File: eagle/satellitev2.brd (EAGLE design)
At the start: 85.1 x 49.5 mm, 12 parts, among them J1 RJ11-6PTH

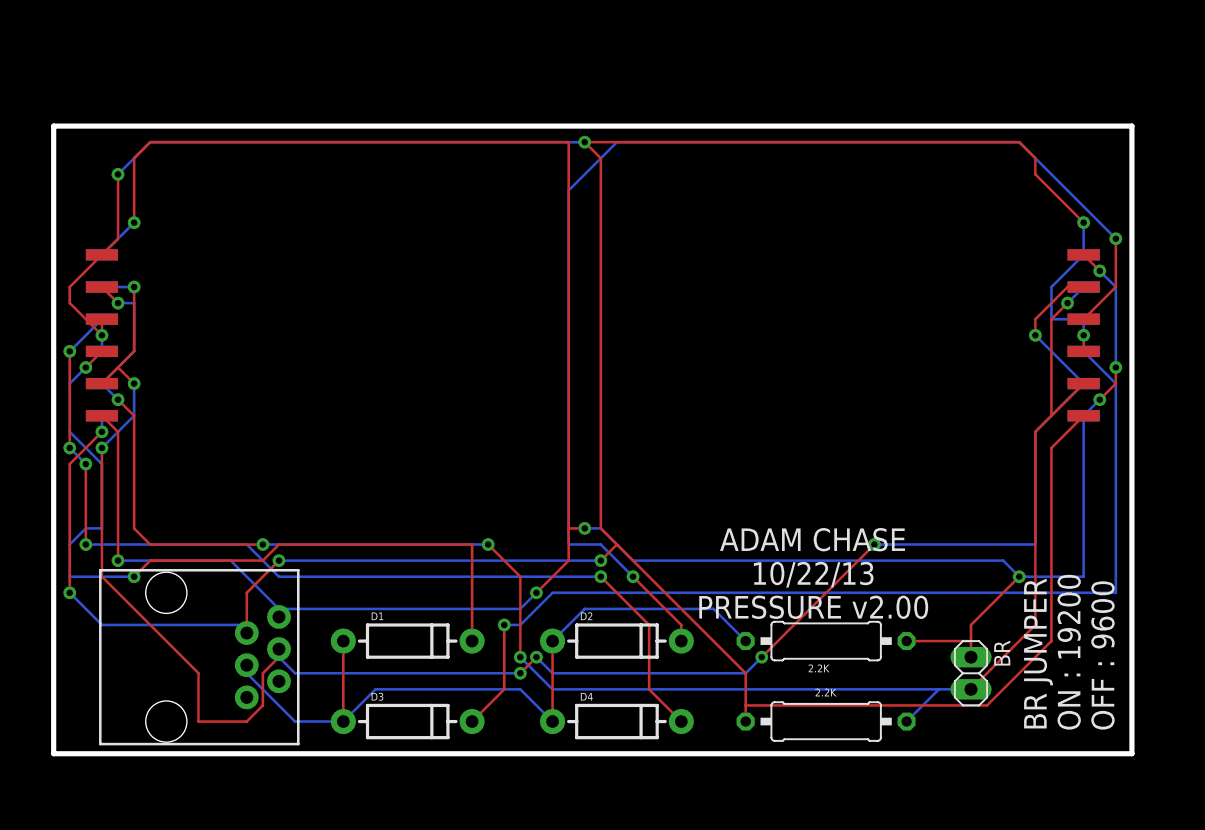
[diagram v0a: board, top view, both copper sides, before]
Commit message: in middle of writing for AIAA paper
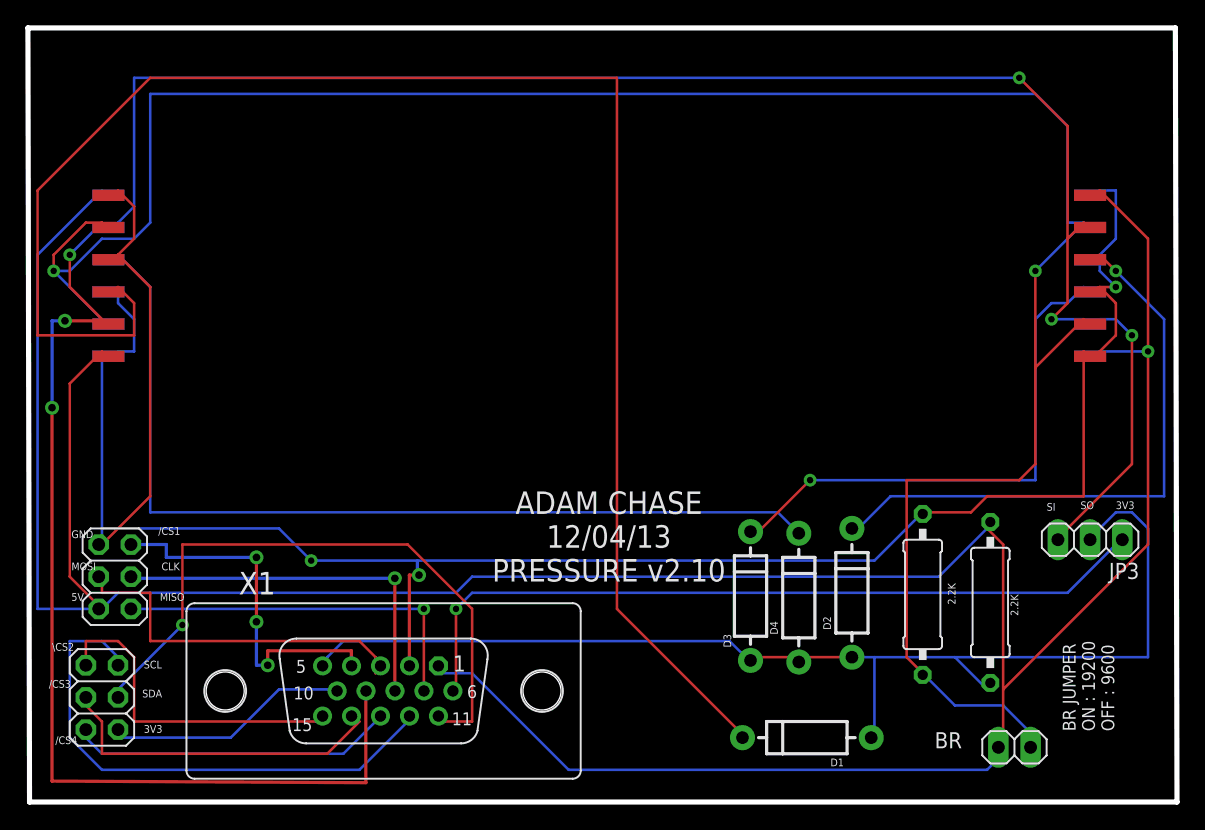
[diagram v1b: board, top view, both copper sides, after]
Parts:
- removed J1: RJ11-6PTH, SparkFun-Connectors:RJ11-6
- added JP1, JP2: (no value), pinhead:2X03
- added JP3: (no value), pinhead:1X03
- added X1: (no value), con-subd:HDF15V
- moved D1 32.4 mm to (59.4, 1.27), turned to 180 degrees
- moved D3 28.8 mm to (55.0, 12.4), turned to 90 degrees
- moved D2 18.9 mm to (63.0, 12.7), turned to 90 degrees
- moved D4 17.4 mm to (58.8, 12.3), turned to 90 degrees
- moved R1 13.3 mm to (73.9, 11.9), turned to 270 degrees
- moved R2 12.6 mm to (68.6, 12.6), turned to 270 degrees
- moved BR 6.77 mm to (75.8, 0.51), turned to 0 degrees
- moved U$1 4.73 mm to (4.32, 44.1)
- moved U$2 4.73 mm to (81.8, 44.1)
- moved U$3 4.73 mm to (80.5, 44.1)
- moved U$4 4.73 mm to (3.05, 44.1)
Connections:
- new net 3V3: JP3.1, X1.6
- new net ACCEL2CS: JP1.5, X1.4
- new net D46: JP2.2, X1.13
- new net D47: JP2.4, X1.14
- new net D48: JP2.6, X1.15
- new net MISO: JP1.1, X1.7
- new net MOSI: JP1.4, X1.3
- new net SCL: JP2.5, X1.12
- new net SCLK: JP1.3, X1.8
- new net SDA: JP2.3, X1.11
- new net TEMPBUS: JP2.1, X1.10
- net 5V: now also JP1.2, X1.1; no longer J1.1
- net GND: now also JP1.6, X1.2; no longer J1.2
- net RX: now also JP3.3, X1.9; no longer J1.3
- net TX: now also JP3.2, X1.5; no longer J1.4
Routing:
- net GND: track 272.9 -> 181.2 mm, vias 9 -> 3
- net RX: track 146.4 -> 215.9 mm, vias 8 -> 6
- net N$2: track 62.1 -> 130.2 mm, vias 2 -> 0
- net 3V3: track 0.00 -> 61.4 mm, vias 0 -> 1
- net SDA: track 0.00 -> 51.0 mm, vias 0 -> 1
- net N$1: track 96.0 -> 47.7 mm, vias 2 -> 1
- net 5V: track 210.5 -> 256.2 mm, vias 8 -> 1
- net SCL: track 0.00 -> 42.3 mm
- net BR: track 140.6 -> 180.3 mm, vias 6 -> 2
- net N$4: track 78.1 -> 42.3 mm
- net TX: track 58.5 -> 93.9 mm
- net SCLK: track 0.00 -> 29.9 mm, vias 0 -> 1
- net MISO: track 0.00 -> 29.6 mm, vias 0 -> 1
- net MOSI: track 0.00 -> 29.4 mm
- net ACCEL2CS: track 0.00 -> 29.3 mm, vias 0 -> 3
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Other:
- board size 85.1 x 49.5 mm -> 90.7 x 61.1 mm
- board text added: "/CS1"
- board text added: "/CS3"
- board text added: "/CS4"
- board text added: "3V3"
- board text added: "ADAM CHASE 12/04/13 PRESSURE v2.10"
- board text added: "CLK"
- board text added: "MISO"
- board text added: "MOSI"
- board text added: "SCL"
- board text added: "SDA"
- board text added: "\CS2"
- board text removed: "ADAM CHASE 10/22/13 PRESSURE v2.00"

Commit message: modified eagle boards and ordered.
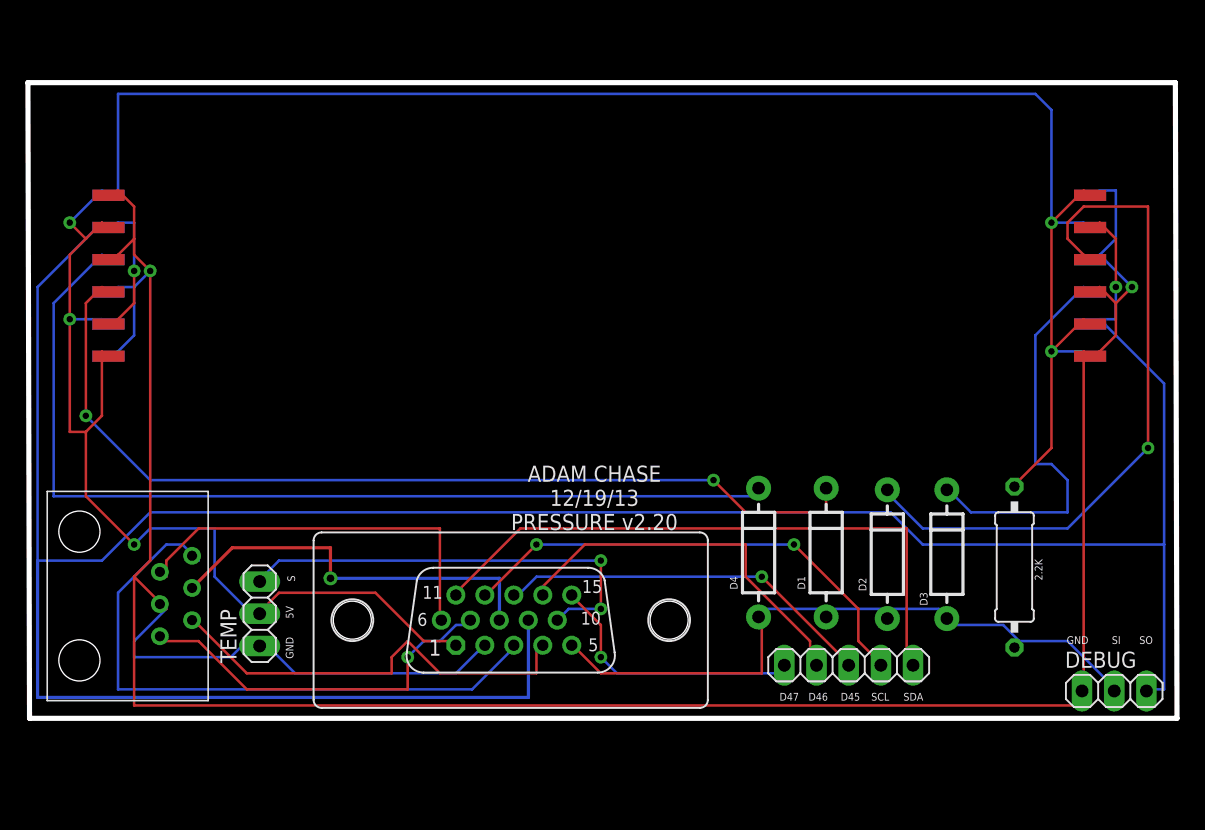
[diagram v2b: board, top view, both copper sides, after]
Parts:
- removed BR: (no value), pinhead:1X02
- removed JP2: (no value), pinhead:2X03
- removed JP3: (no value), pinhead:1X03
- removed R2: 2.2K, rcl:0309/12
- added DEBUG, TEMP: (no value), pinhead:1X03
- added U$5: RJ11V, RJ11V:RJ11V
- JP1: device pinhead:2X03 -> pinhead:1X05
- moved JP1 58.3 mm to (62.7, 6.99), turned to 180 degrees
- moved D3 15.8 mm to (70.5, 15.7)
- moved D1 14.7 mm to (61.0, 15.9), turned to 90 degrees
- moved X1 11.5 mm to (36.1, 10.5), turned to 180 degrees
- moved D4 4.77 mm to (55.6, 15.9)
- moved D2 4.13 mm to (65.8, 15.7)
- moved R1 3.38 mm to (75.8, 14.7)
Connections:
- removed net BR: BR.2, R2.2, U$1.P$2, U$2.P$5, U$3.P$2, U$4.P$5
- removed net D48: JP2.6, X1.15
- new net D45: JP1.3, X1.13
- net 3V3: now also U$5.P$6; no longer JP3.1
- net 5V: now also TEMP.2, U$1.P$2, U$2.P$5, U$3.P$2, U$4.P$5; no longer BR.1, JP1.2
- net ACCEL2CS: now also U$5.P$1; no longer JP1.5
- net D46: now also JP1.4, X1.14; no longer JP2.2, X1.13
- net D47: now also JP1.5, X1.15; no longer JP2.4, X1.14
- net GND: now also DEBUG.1, TEMP.1, U$5.P$5; no longer JP1.6, R2.1
- net MISO: now also U$5.P$4; no longer JP1.1
- net MOSI: now also U$5.P$3; no longer JP1.4
- net RX: now also DEBUG.3; no longer JP3.3
- net SCL: now also JP1.2; no longer JP2.5
- net SCLK: now also U$5.P$2; no longer JP1.3
- net SDA: now also JP1.1; no longer JP2.3
- net TEMPBUS: now also TEMP.3; no longer JP2.1
- net TX: now also DEBUG.2; no longer JP3.2
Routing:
- net BR: track 180.3 -> 0.00 mm, vias 2 -> 0
- net N$2: track 130.2 -> 74.8 mm, vias 0 -> 2
- net 5V: track 256.2 -> 208.5 mm, vias 1 -> 5
- net GND: track 181.2 -> 222.5 mm, vias 3 -> 2
- net TX: track 93.9 -> 54.7 mm
- net D45: track 0.00 -> 29.9 mm, vias 0 -> 1
- net 3V3: track 61.4 -> 32.6 mm, vias 1 -> 0
- net D48: track 27.1 -> 0.00 mm
- net MOSI: track 29.4 -> 50.7 mm
- net TEMPBUS: track 20.5 -> 36.3 mm, vias 0 -> 2
- net RX: track 215.9 -> 231.6 mm, vias 6 -> 2
- net N$4: track 42.3 -> 32.0 mm, vias 1 -> 0
- net N$1: track 47.7 -> 54.2 mm
- net ACCEL2CS: track 29.3 -> 34.9 mm, vias 3 -> 0
- net D47: track 27.1 -> 21.7 mm, vias 0 -> 1
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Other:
- board size 90.7 x 61.1 mm -> 90.7 x 50.2 mm
- board text added: "ADAM CHASE 12/19/13 PRESSURE v2.20"
- board text added: "D45"
- board text added: "D46"
- board text added: "D47"
- board text added: "S"
- board text removed: "/CS1"
- board text removed: "/CS3"
- board text removed: "/CS4"
- board text removed: "3V3"
- board text removed: "ADAM CHASE 12/04/13 PRESSURE v2.10"
- board text removed: "BR JUMPER ON : 19200 OFF : 9600"
- board text removed: "CLK"
- board text removed: "MISO"
- board text removed: "MOSI"
- board text removed: "\CS2"
